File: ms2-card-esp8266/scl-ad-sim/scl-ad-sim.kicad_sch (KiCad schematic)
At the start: 7 parts, among them Q1 MMBT5401

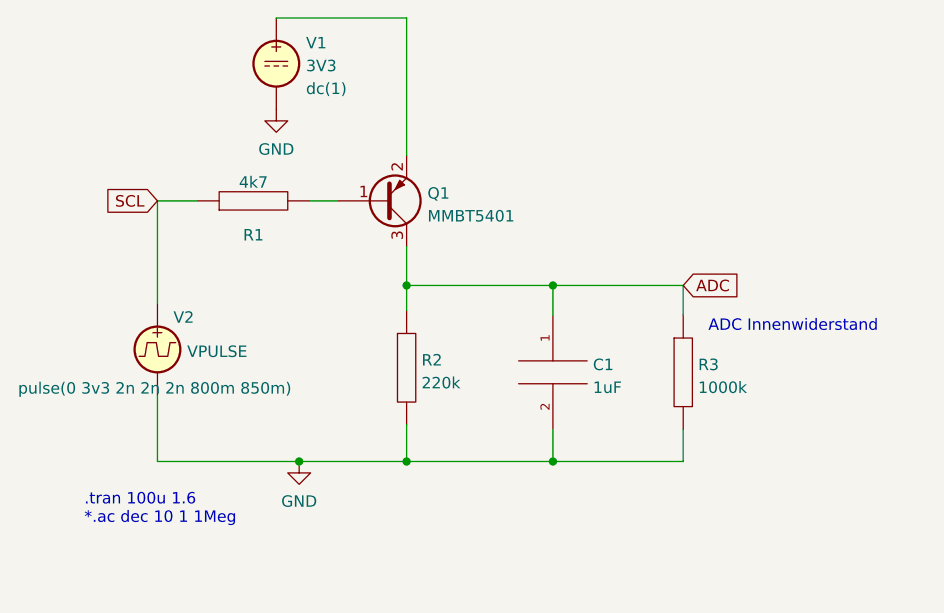
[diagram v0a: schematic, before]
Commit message: use JLCPCB standard parts
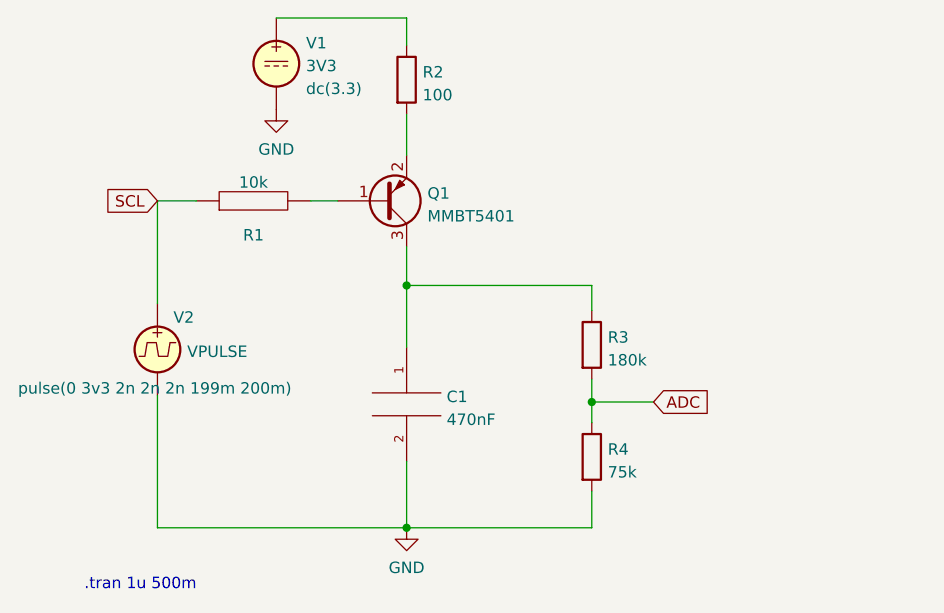
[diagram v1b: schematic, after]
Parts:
- removed R2: 220k, symbol pspice:R
- removed R3: 1000k, symbol pspice:R
- added R2: 100, symbol Device:R
- added R3: 180k, symbol Device:R
- added R4: 75k, symbol Device:R
- C1: value 1uF -> 470nF
- Q1: Spice_Node_Sequence 2 1 3 -> 3 1 2
- R1: value 4k7 -> 10k
- V1: Spice_Model dc(1) -> dc(3.3)
- V2: Spice_Model pulse(0 3v3 2n 2n 2n 800m 850m) -> pulse(0 3v3 2n 2n 2n 199m 200m)
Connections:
- net ADC: now also R3.2, R4.1; no longer C1.1, Q1.3 (C)
- net GND: now also R4.2
- net at Q1.2 (E): now also R2.2; no longer V1.1
- new net: C1.1, Q1.3 (C), R3.1
- new net: R2.1, V1.1
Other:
- note added: ".tran 1u 500m"
- note removed: ".tran 100u 1.6 *.ac dec 10 1 1Meg"
- note removed: "ADC Innenwiderstand"
- moved on the sheet: C1
